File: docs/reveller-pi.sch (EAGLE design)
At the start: 21 parts, among them Q2 BS270, T1 BC547, X1 CANTON-POWER, X2 RASPI_BOARD_AB_E0, X3 PG203J

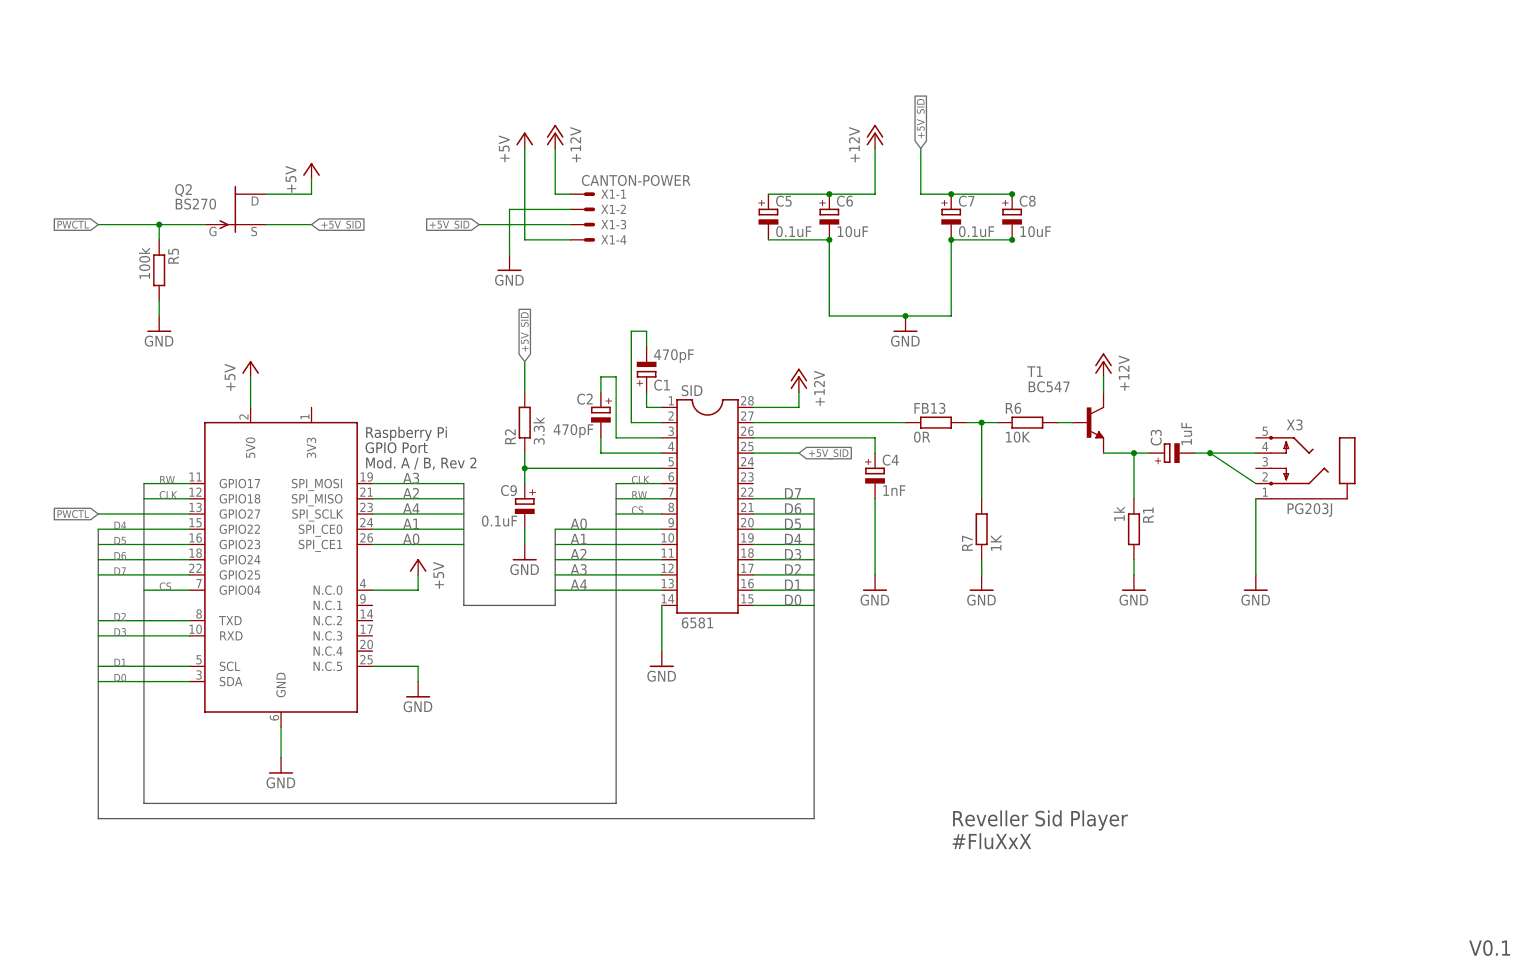
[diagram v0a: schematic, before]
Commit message: Completed powercontrol and boarddesign
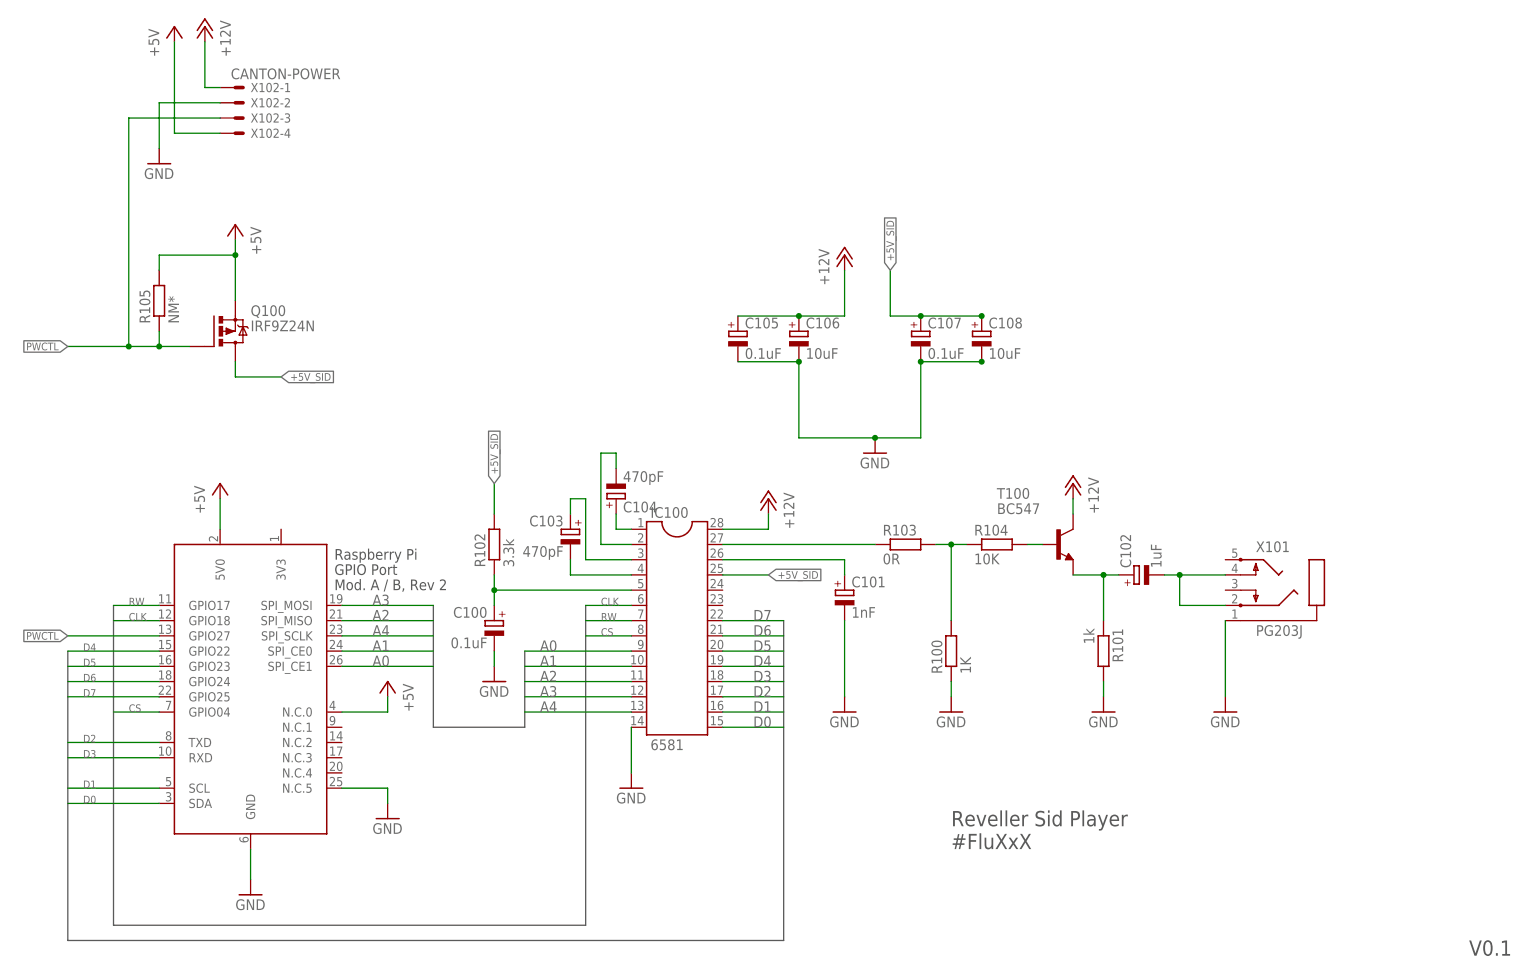
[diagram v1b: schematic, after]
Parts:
- removed C1, C2: 470pF, rcl:CPOL-EUE2.5-5
- removed C3: 1uF, rcl:CPOL-EUE2.5-5
- removed C4: 1nF, rcl:CPOL-EUE2.5-5
- removed C5, C7, C9: 0.1uF, rcl:CPOL-EUE2.5-5
- removed C6, C8: 10uF, rcl:CPOL-EUE2.5-5
- removed FB13: 0R, rcl:R-EU_0204/7
- removed Q2: BS270, transistor-fet:2N5484
- removed R1: 1k, rcl:R-EU_0204/7
- removed R2: 3.3k, rcl:R-EU_0204/7
- removed R5: 100k, rcl:R-EU_0204/7
- removed R6: 10K, rcl:R-EU_0204/7
- removed R7: 1K, rcl:R-EU_0204/7
- removed SID: 6581, ic-package:DIL28
- removed T1: BC547, transistor:BC547
- removed X1: CANTON-POWER, con-molex:22-23-2041
- removed X2: RASPI_BOARD_AB_E0, raspberrypi_bastelstube_v13:RASPI_BOARD_AB_E0
- removed X3: PG203J, con-hirschmann:PG203J
- added C100, C105, C107: 0.1uF, rcl:CPOL-EUE2.5-5
- added C101: 1nF, rcl:CPOL-EUE2.5-5
- added C102: 1uF, rcl:CPOL-EUE2.5-5
- added C103, C104: 470pF, rcl:CPOL-EUE2.5-5
- added C106, C108: 10uF, rcl:CPOL-EUE2.5-5
- added IC100: 6581, ic-package:DIL28
- added Q100: IRF9Z24N, transistor-power:IRF9530
- added R100: 1K, rcl:R-EU_0204/7
- added R101: 1k, rcl:R-EU_0204/7
- added R102: 3.3k, rcl:R-EU_0204/7
- added R103: 0R, rcl:R-EU_0204/7
- added R104: 10K, rcl:R-EU_0204/7
- added R105: NM*, rcl:R-EU_0204/7
- added T100: BC547, transistor:BC547
- added X100: RASPI_BOARD_AB_E0, raspberrypi_bastelstube_v13:RASPI_BOARD_AB_E0
- added X101: PG203J, con-hirschmann:PG203J
- added X102: CANTON-POWER, con-molex:22-23-2041
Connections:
- net +12V: now also C105.+, C106.+, IC100.28, T100.C, X102-1.S; no longer C5.+, C6.+, SID.28, T1.C, X1-1.S
- net +5V: now also Q100.S, R105.2, X100.5V0, X100.N.C.0, X102-4.S; no longer Q2.D, X1-4.S, X2.5V0, X2.N.C.0
- net +5V_SID: now also C107.+, C108.+, IC100.25, Q100.D, R102.2; no longer C7.+, C8.+, Q2.S, R2.2, SID.25, X1-3.S
- net A0: now also IC100.9, X100.SPI_CE1; no longer SID.9, X2.SPI_CE1
- net A1: now also IC100.10, X100.SPI_CE0; no longer SID.10, X2.SPI_CE0
- net A2: now also IC100.11, X100.SPI_MISO; no longer SID.11, X2.SPI_MISO
- net A3: now also IC100.12, X100.SPI_MOSI; no longer SID.12, X2.SPI_MOSI
- net A4: now also IC100.13, X100.SPI_SCLK; no longer SID.13, X2.SPI_SCLK
- net AUDIO_DC: now also C102.+, R101.1, T100.E; no longer C3.+, R1.1, T1.E
- net AUDIO_OUT: now also C102.-, X101.2, X101.4; no longer C3.-, X3.2, X3.4
- net AUDIO_PREAMP: now also R100.2, R103.2, R104.1; no longer FB13.2, R6.1, R7.2
- net AUDIO_PREAMP_B: now also R104.2, T100.B; no longer R6.2, T1.B
- net AUDIO_RAW: now also IC100.27, R103.1; no longer FB13.1, SID.27
- net CAP1A: now also C104.+, IC100.1; no longer C1.+, SID.1
- net CAP1B: now also C104.-, IC100.2; no longer C1.-, SID.2
- net CAP2A: now also C103.+, IC100.3; no longer C2.+, SID.3
- net CAP2B: now also C103.-, IC100.4; no longer C2.-, SID.4
- net CAPX: now also C101.+, IC100.26; no longer C4.+, SID.26
- net CLK: now also IC100.6, X100.GPIO18; no longer SID.6, X2.GPIO18
- net CS: now also IC100.8, X100.GPIO04; no longer SID.8, X2.GPIO04
- net D0: now also IC100.15, X100.SDA; no longer SID.15, X2.SDA
- net D1: now also IC100.16, X100.SCL; no longer SID.16, X2.SCL
- net D2: now also IC100.17, X100.TXD; no longer SID.17, X2.TXD
- net D3: now also IC100.18, X100.RXD; no longer SID.18, X2.RXD
- net D4: now also IC100.19, X100.GPIO22; no longer SID.19, X2.GPIO22
- net D5: now also IC100.20, X100.GPIO23; no longer SID.20, X2.GPIO23
- net D6: now also IC100.21, X100.GPIO24; no longer SID.21, X2.GPIO24
- net D7: now also IC100.22, X100.GPIO25; no longer SID.22, X2.GPIO25
- net GND: now also C100.-, C101.-, C105.-, C106.-, C107.-, C108.-, IC100.14, R100.1, R101.2, X100.GND, X100.N.C.5, X101.1, X102-2.S; no longer C4.-, C5.-, C6.-, C7.-, C8.-, C9.-, R1.2, R5.2, R7.1, SID.14, X1-2.S, X2.GND, X2.N.C.5, X3.1
- net PWCTL: now also Q100.G, R105.1, X100.GPIO27, X102-3.S; no longer Q2.G, R5.1, X2.GPIO27
- net RESET: now also C100.+, IC100.5, R102.1; no longer C9.+, R2.1, SID.5
- net RW: now also IC100.7, X100.GPIO17; no longer SID.7, X2.GPIO17
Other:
- note added: "* R105 is present inside the canton power module, so no need for it here"
- note added: "PWCTL: low=on high/open=off"
